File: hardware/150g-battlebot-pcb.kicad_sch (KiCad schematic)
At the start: 0 parts

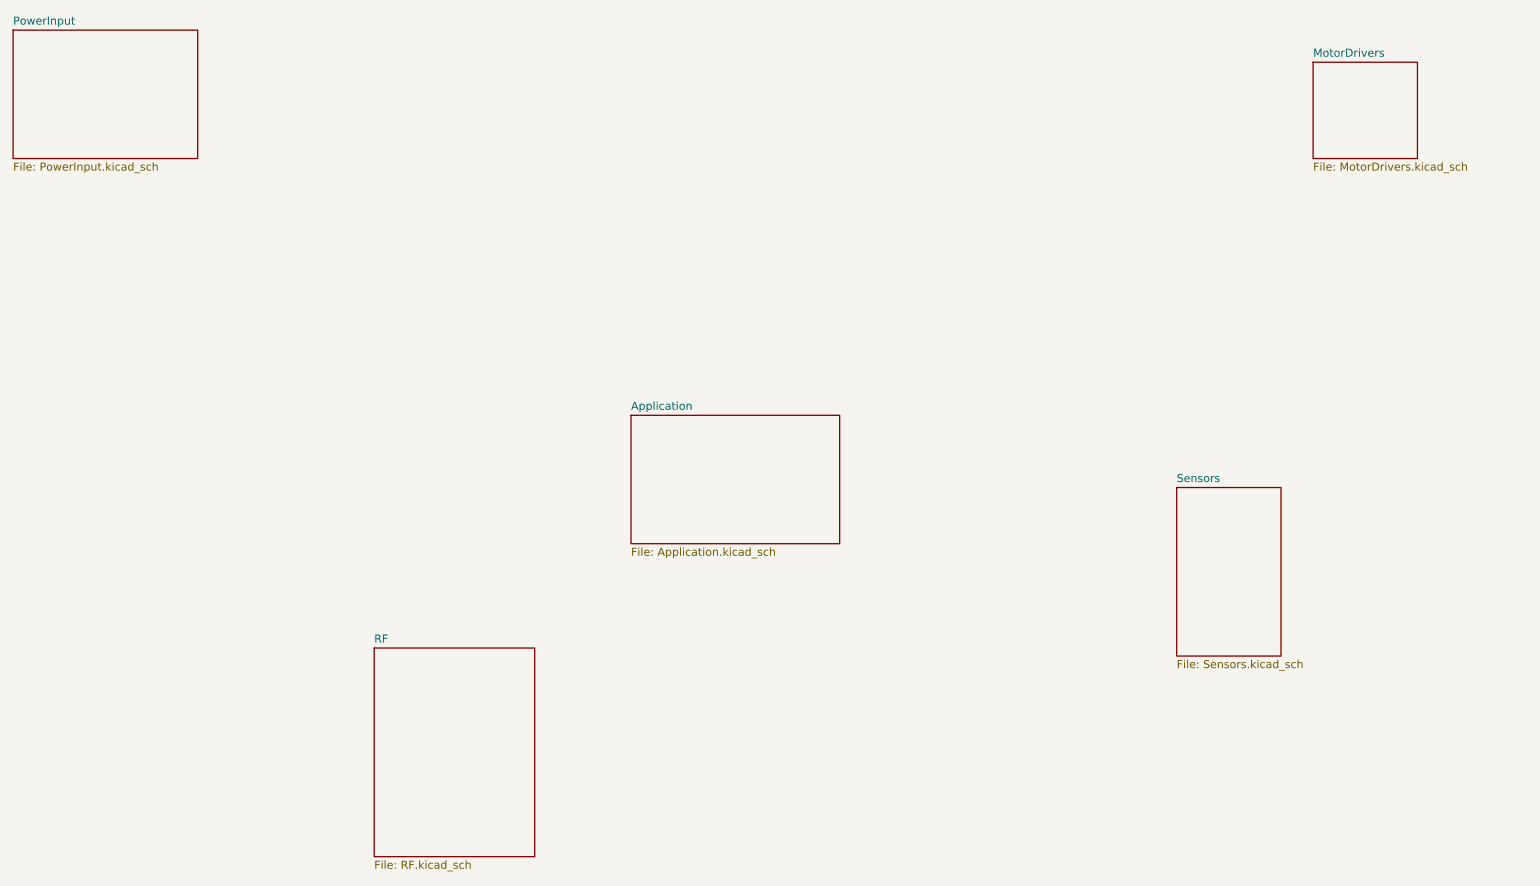
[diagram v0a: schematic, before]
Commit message: asdf
Signed-off-by: Connor Rigby <connorr@hey.com>
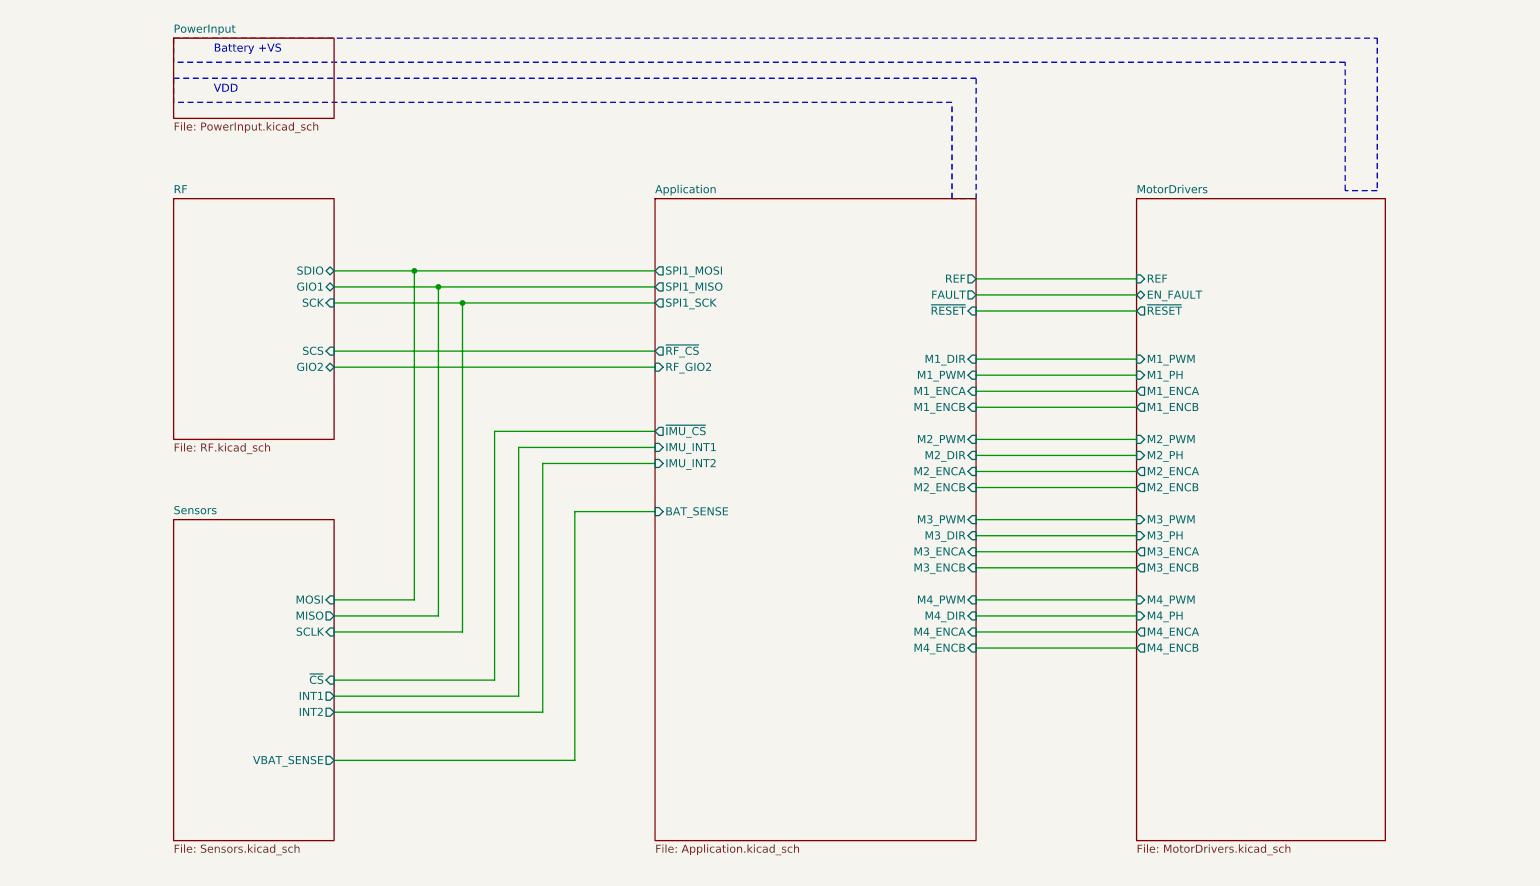
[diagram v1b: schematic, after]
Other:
- sheet Application ports: added BAT_SENSE, FAULT, IMU_INT1, IMU_INT2, M1_DIR, M1_ENCA, M1_ENCB, M1_PWM, M2_DIR, M2_ENCA, M2_ENCB, M2_PWM, M3_DIR, M3_ENCA, M3_ENCB, M3_PWM, M4_DIR, M4_ENCA, M4_ENCB, M4_PWM, REF, RF_GIO2, SPI1_MISO, SPI1_MOSI, SPI1_SCK, ~{IMU_CS}, ~{RESET}, ~{RF_CS}; removed none
- sheet MotorDrivers ports: added EN_FAULT, M1_ENCA, M1_ENCB, M1_PH, M1_PWM, M2_ENCA, M2_ENCB, M2_PH, M2_PWM, M3_ENCA, M3_ENCB, M3_PH, M3_PWM, M4_ENCA, M4_ENCB, M4_PH, M4_PWM, REF, ~{RESET}; removed none
- sheet RF ports: added GIO1, GIO2, SCK, SCS, SDIO; removed none
- sheet Sensors ports: added INT1, INT2, MISO, MOSI, SCLK, VBAT_SENSE, ~{CS}; removed none
- note added: "Battery +VS"
- note added: "VDD"
